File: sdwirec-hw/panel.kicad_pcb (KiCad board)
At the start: 4 copper layers, 71 x 70 mm, 272 parts, among them IC1 USB2640-HZH-02, IC2 MC74HC1G04DTT1G, J1 USB_C_Receptacle_USB2.0, J2 usd_plug, J3 Micro_SD_Card, Q1 SMMBT4403L, Q2 SMMBT4403L, U1 M24C02-RDW, U2 SPX3819M5-L-3-3, U3 TS3A27518EPW, U4 FT200XD, Y1 24Mhz

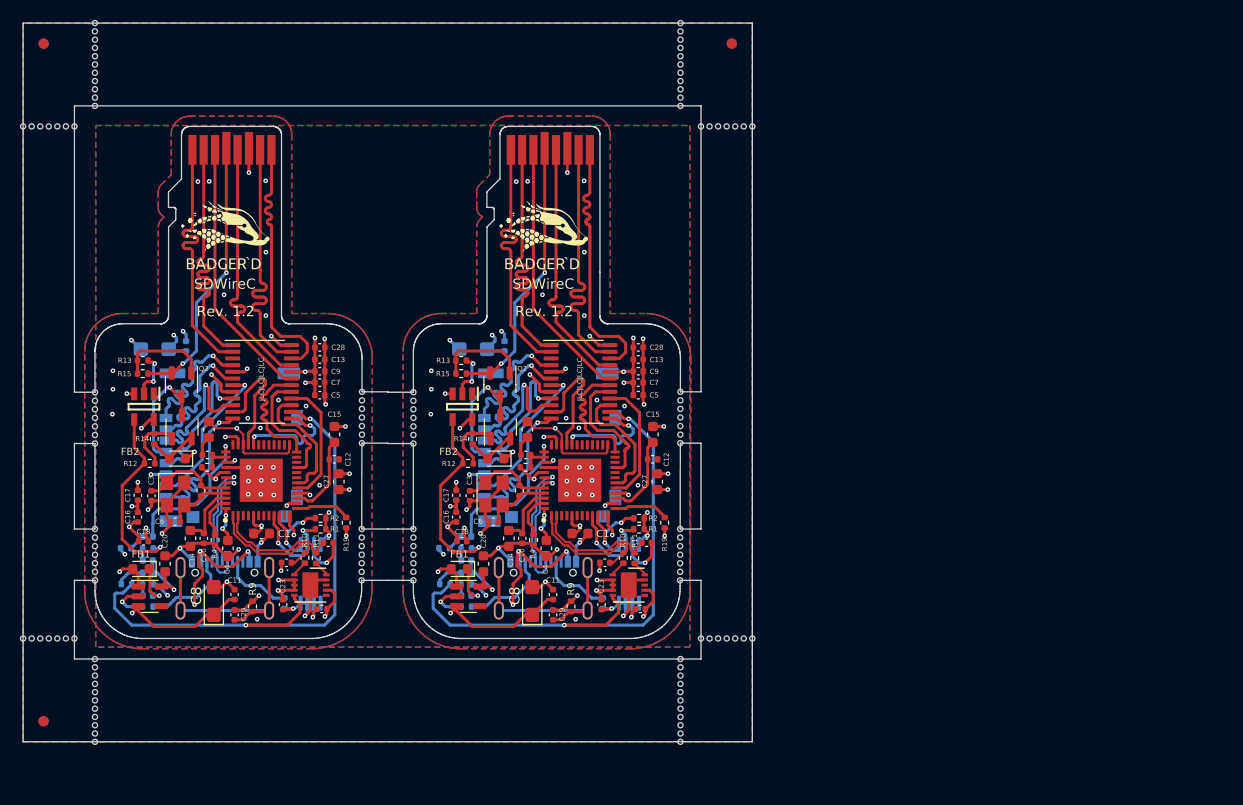
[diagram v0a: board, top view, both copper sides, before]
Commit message: Update to Rev 1.4
Signed-off-by: Talha Can Havadar <talha.can.havadar@canonical.com>
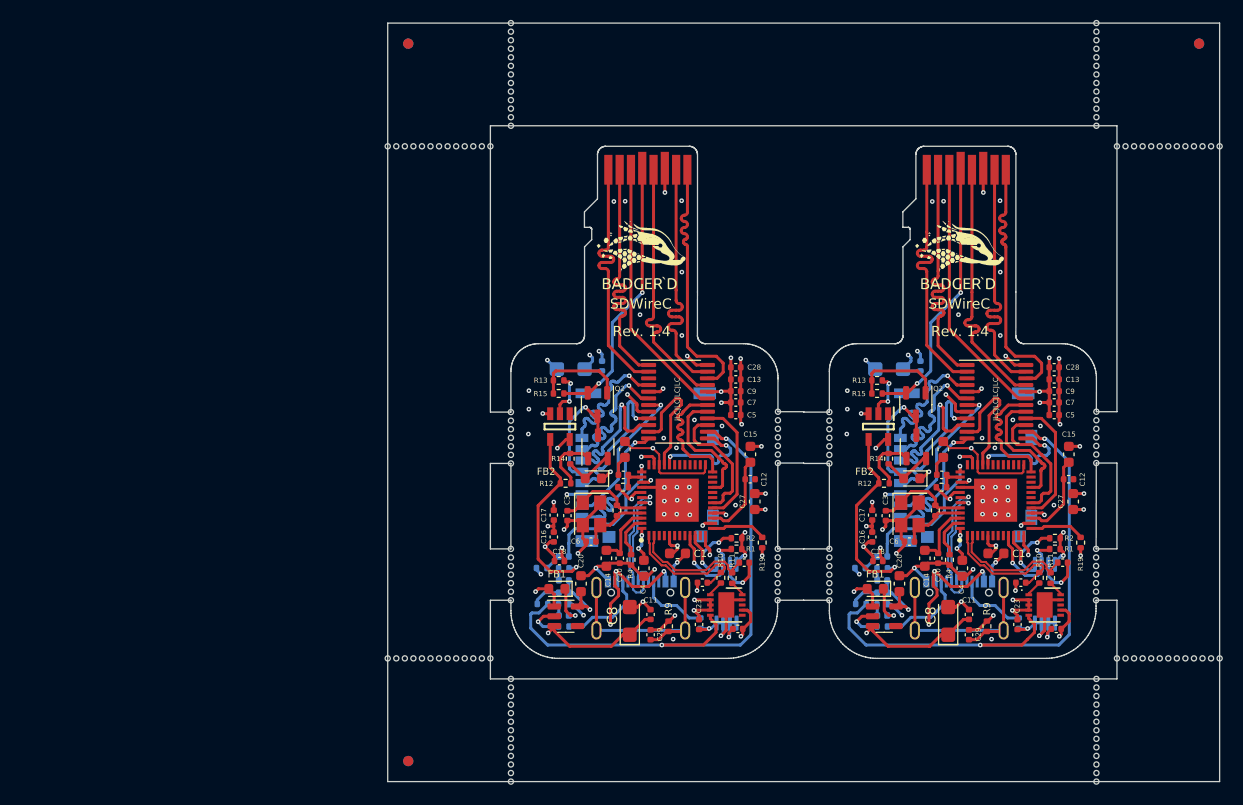
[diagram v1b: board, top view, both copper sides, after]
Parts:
- removed the C1 at (167.2, 69.7)
- removed the C1 at (136.2, 69.7)
- removed the C10 at (130.6, 70.2)
- removed the C10 at (161.6, 70.2)
- removed the C11 at (133.6, 75.7)
- removed the C11 at (164.6, 75.7)
- removed the C12 at (143.3, 62.5)
- removed the C12 at (174.3, 62.5)
- removed the C13 at (141.9, 52.8)
- removed the C13 at (172.9, 52.8)
- removed the C14 at (129.3, 70.2)
- removed the C14 at (160.3, 70.2)
- removed the C15 at (143.3, 60.1)
- removed the C15 at (174.3, 60.1)
- removed the C16 at (124.2, 68.1)
- removed the C16 at (155.2, 68.1)
- removed the C17 at (124.2, 66.0)
- removed the C17 at (155.2, 66.0)
- removed the C18 at (124.7, 70.5)
- removed the C18 at (155.7, 70.5)
- removed the C19 at (130.9, 62.1)
- removed the C19 at (162.0, 62.1)
- removed the C2 at (173.1, 77.1)
- removed the C2 at (142.1, 77.1)
- removed the C20 at (157.8, 72.7)
- removed the C20 at (126.8, 72.7)
- removed the C21 at (169.7, 72.6)
- removed the C21 at (138.6, 72.6)
- removed the C22 at (173.7, 70.6)
- removed the C22 at (142.7, 70.6)
- removed the C23 at (138.3, 76.6)
- removed the C23 at (169.3, 76.6)
- removed the C24 at (125.8, 51.8)
- removed the C24 at (156.8, 51.8)
- removed the C25 at (128.9, 51.5)
- removed the C25 at (159.9, 51.5)
- removed the C26 at (162.1, 59.6)
- removed the C26 at (131.1, 59.6)
- removed the C27 at (174.8, 64.7)
- removed the C27 at (143.7, 64.7)
- removed the C28 at (172.9, 51.6)
- removed the C28 at (141.9, 51.6)
- removed the C29 at (133.6, 77.6)
- removed the C29 at (164.6, 77.6)
- removed the C3 at (156.5, 66.0)
- removed the C3 at (125.5, 66.0)
- removed the C4 at (132.9, 71.2)
- removed the C4 at (164.0, 71.2)
- removed the C5 at (172.9, 56.2)
- removed the C5 at (141.9, 56.2)
- removed the C6 at (127.8, 68.6)
- removed the C6 at (158.8, 68.6)
- removed the C7 at (172.9, 55.0)
- removed the C7 at (141.9, 55.0)
- removed the C8 at (162.6, 76.3)
- removed the C8 at (131.6, 76.3)
- removed the C9 at (172.9, 53.9)
- removed the C9 at (141.9, 53.9)
- removed the D1 at (125.1, 75.8)
- removed the D1 at (156.2, 75.8)
- removed the D2 at (156.2, 70.0)
- removed the D2 at (125.1, 70.0)
- removed the D3 at (156.2, 73.5)
- removed the D3 at (125.1, 73.5)
- removed the D4 at (156.2, 72.3)
- removed the D4 at (125.1, 72.3)
- removed the FB1 at (155.5, 73.2)
- removed the FB1 at (124.5, 73.2)
- removed the FB2 at (159.0, 62.4)
- removed the FB2 at (128.0, 62.4)
- removed the G*** at (132.7, 40.7) (x2)
- removed the G*** at (163.7, 40.7) (x2)
- removed the IC1 at (136.2, 64.5)
- removed the IC1 at (167.2, 64.5)
- removed the IC2 at (124.8, 57.4)
- removed the IC2 at (155.8, 57.4)
- removed the J1 at (163.7, 76.1)
- removed the J1 at (132.6, 76.1)
- removed the J2 at (160.5, 32.3)
- removed the J2 at (129.5, 32.3)
- removed the J3 at (158.6, 61.3)
- removed the J3 at (127.5, 61.3)
- removed the Q1 at (159.5, 59.3)
- removed the Q1 at (128.5, 59.3)
- removed the Q2 at (128.4, 55.2)
- removed the Q2 at (159.4, 55.2)
- removed the R1 at (173.0, 69.3)
- removed the R1 at (142.0, 69.3)
- removed the R10 at (140.4, 72.1)
- removed the R10 at (171.5, 72.1)
- removed the R11 at (141.5, 72.1)
- removed the R11 at (172.6, 72.1)
- removed the R12 at (156.3, 62.9)
- removed the R12 at (125.3, 62.9)
- removed the R13 at (155.7, 52.9)
- removed the R13 at (124.6, 52.9)
- removed the R14 at (156.8, 60.5)
- removed the R14 at (125.8, 60.5)
- removed the R15 at (124.6, 54.1)
- removed the R15 at (155.7, 54.1)
- removed the R16 at (154.1, 74.6)
- removed the R16 at (123.1, 74.6)
- removed the R17 at (125.1, 71.2)
- removed the R17 at (156.2, 71.2)
- removed the R18 at (161.3, 65.5)
- removed the R18 at (130.3, 65.5)
- removed the R19 at (144.5, 68.7)
- removed the R19 at (175.5, 68.7)
- removed the R2 at (173.0, 68.2)
- removed the R2 at (142.0, 68.2)
- removed the R3 at (125.1, 74.7)
- removed the R3 at (156.2, 74.7)
- removed the R4 at (131.7, 70.3)
- removed the R4 at (162.7, 70.3)
- removed the R5 at (161.9, 63.3)
- removed the R5 at (130.9, 63.3)
- removed the R6 at (154.0, 71.1)
- removed the R6 at (123.0, 71.1)
- removed the R7 at (125.1, 76.8)
- removed the R7 at (156.2, 76.8)
- removed the R8 at (169.5, 76.5)
- removed the R8 at (138.4, 76.5)
- removed the R9 at (166.4, 76.8)
- removed the R9 at (135.3, 76.8)
- removed the REF** at (120.0, 82.7)
- removed the REF** at (177.0, 60.9)
- removed the REF** at (117.2, 30.1)
- removed the REF** at (177.0, 73.4)
- removed the REF** at (177.0, 24.8)
- removed the REF** at (177.0, 81.9)
- removed the REF** at (151.0, 60.1)
- removed the REF** at (182.3, 30.1)
- removed the REF** at (177.0, 82.7)
- removed the REF** at (182.0, 22.0) (x2)
- removed the REF** at (177.0, 69.3)
- removed the REF** at (120.0, 56.0)
- removed the REF** at (151.0, 70.1)
- removed the REF** at (120.0, 23.2)
- removed the REF** at (120.0, 74.3)
- removed the REF** at (184.0, 79.9)
- removed the REF** at (120.0, 28.1)
- removed the REF** at (177.0, 84.4)
- removed the REF** at (120.0, 83.5)
- removed the REF** at (151.0, 73.4)
- removed the REF** at (179.8, 30.1)
- removed the REF** at (120.0, 84.4)
- removed the REF** at (177.0, 20.0)
- removed the REF** at (146.0, 73.4)
- removed the REF** at (120.0, 58.5)
- removed the REF** at (177.0, 57.6)
- removed the REF** at (177.0, 24.0)
- removed the REF** at (180.7, 30.1)
- removed the REF** at (146.0, 74.3)
- removed the REF** at (120.0, 21.6)
- removed the REF** at (177.0, 27.3)
- removed the REF** at (177.0, 72.6)
- removed the REF** at (120.0, 27.3)
- removed the REF** at (120.0, 86.0)
- removed the REF** at (182.3, 79.9)
- removed the REF** at (146.0, 57.6)
- removed the REF** at (177.0, 21.6)
- removed the REF** at (133.8, 50.2)
- removed the REF** at (115.0, 22.0) (x2)
- removed the REF** at (115.0, 88.0) (x2)
- removed the REF** at (164.8, 50.2)
- removed the REF** at (177.0, 55.9)
- removed the REF** at (177.0, 89.2)
- removed the REF** at (177.0, 26.4)
- removed the REF** at (183.2, 79.9)
- removed the REF** at (120.0, 56.8)
- removed the REF** at (118.0, 30.1)
- removed the REF** at (117.2, 79.9)
- removed the REF** at (120.0, 86.8)
- removed the REF** at (146.0, 72.6)
- removed the REF** at (120.0, 81.9)
- removed the REF** at (177.0, 25.6)
- removed the REF** at (120.0, 24.8)
- removed the REF** at (177.0, 22.4)
- removed the REF** at (151.0, 71.8)
- removed the REF** at (120.0, 87.6)
- removed the REF** at (146.0, 70.1)
- removed the REF** at (120.0, 25.6)
- removed the REF** at (181.5, 79.9)
- removed the REF** at (120.0, 22.4)
- removed the REF** at (151.0, 57.6)
- removed the REF** at (177.0, 70.9)
- removed the REF** at (177.0, 86.0)
- removed the REF** at (177.0, 28.1)
- removed the REF** at (151.0, 74.3)
- removed the REF** at (114.7, 30.1)
- removed the REF** at (114.7, 79.9)
- removed the REF** at (120.0, 70.1)
- removed the REF** at (113.8, 30.1)
- removed the REF** at (120.0, 57.6)
- removed the REF** at (113.0, 79.9)
- removed the REF** at (120.0, 85.2)
- removed the REF** at (151.0, 56.8)
- removed the REF** at (179.0, 30.1)
- removed the REF** at (177.0, 85.2)
- removed the REF** at (183.2, 30.1)
- removed the REF** at (146.0, 56.7)
- removed the REF** at (120.0, 24.0)
- removed the REF** at (120.0, 59.3)
- removed the REF** at (177.0, 59.2)
- removed the REF** at (151.0, 58.5)
- removed the REF** at (177.0, 87.6)
- removed the REF** at (177.0, 58.4)
- removed the REF** at (179.8, 79.9)
- removed the REF** at (177.0, 56.7)
- removed the REF** at (120.0, 26.4)
- removed the REF** at (180.7, 79.9)
- removed the REF** at (120.0, 72.6)
- removed the REF** at (177.0, 83.5)
- removed the REF** at (177.0, 90.0)
- removed the REF** at (120.0, 60.1)
- removed the REF** at (146.0, 55.9)
- removed the REF** at (184.0, 30.1)
- removed the REF** at (177.0, 70.1)
- removed the REF** at (146.0, 70.9)
- removed the REF** at (113.0, 30.1)
- removed the REF** at (118.0, 79.9)
- removed the REF** at (146.0, 69.3)
- removed the REF** at (120.0, 89.2)
- removed the REF** at (146.0, 60.1)
- removed the REF** at (177.0, 60.1)
- removed the REF** at (181.5, 30.1)
- removed the REF** at (151.0, 56.0)
- removed the REF** at (146.0, 58.4)
- removed the REF** at (120.0, 90.0)
- removed the REF** at (151.0, 69.3)
- removed the REF** at (115.5, 30.1)
- removed the REF** at (177.0, 23.2)
- removed the REF** at (151.0, 70.9)
- removed the REF** at (120.0, 69.3)
- removed the REF** at (120.0, 20.0)
- removed the REF** at (120.0, 73.4)
- removed the REF** at (120.0, 88.4)
- removed the REF** at (146.0, 59.2)
- removed the REF** at (151.0, 72.6)
- removed the REF** at (113.8, 79.9)
- removed the REF** at (120.0, 20.8)
- removed the REF** at (177.0, 86.8)
- removed the REF** at (116.3, 30.1)
- removed the REF** at (116.3, 79.9)
- removed the REF** at (115.5, 79.9)
- removed the REF** at (177.0, 20.8)
- removed the REF** at (146.0, 60.9)
- removed the REF** at (120.0, 61.0)
- removed the REF** at (179.0, 79.9)
- removed the REF** at (120.0, 70.9)
- removed the REF** at (151.0, 61.0)
- removed the REF** at (177.0, 74.3)
- removed the REF** at (146.0, 71.8)
- removed the REF** at (177.0, 88.4)
- removed the REF** at (177.0, 71.8)
- removed the REF** at (120.0, 71.8)
- removed the REF** at (151.0, 59.3)
- removed the U1 at (172.0, 73.6)
- removed the U1 at (141.0, 73.6)
- removed the U2 at (125.3, 75.8)
- removed the U2 at (156.4, 75.8)
- removed the U3 at (167.3, 54.9)
- removed the U3 at (136.3, 54.9)
- removed the U4 at (141.0, 74.7)
- removed the U4 at (172.0, 74.7)
- removed the Y1 at (127.8, 65.9)
- removed the Y1 at (158.9, 65.9)
- added C1: 1uF, Capacitor_SMD:C_0603_1608Metric, F.Cu at (207.7, 71.7)
- added C1: 1uF, Capacitor_SMD:C_0603_1608Metric, F.Cu at (176.7, 71.7)
- added C10: 100nF, Capacitor_SMD:C_0402_1005Metric, F.Cu at (202.1, 72.1)
- added C10: 100nF, Capacitor_SMD:C_0402_1005Metric, F.Cu at (171.1, 72.1)
- added C11: 100nF / 16V, Capacitor_SMD:C_0402_1005Metric, F.Cu at (205.1, 77.6)
- added C11: 100nF / 16V, Capacitor_SMD:C_0402_1005Metric, F.Cu at (174.1, 77.6)
- added C12: 100nF, Capacitor_SMD:C_0402_1005Metric, F.Cu at (214.8, 64.4)
- added C12: 100nF, Capacitor_SMD:C_0402_1005Metric, F.Cu at (183.8, 64.4)
- added C13: 100nF, Capacitor_SMD:C_0402_1005Metric, F.Cu at (182.4, 54.7)
- added C13: 100nF, Capacitor_SMD:C_0402_1005Metric, F.Cu at (213.4, 54.7)
- added C14: 1uF, Capacitor_SMD:C_0603_1608Metric, F.Cu at (200.8, 72.1)
- added C14: 1uF, Capacitor_SMD:C_0603_1608Metric, F.Cu at (169.8, 72.1)
- added C15: 1uF, Capacitor_SMD:C_0603_1608Metric, F.Cu at (214.8, 62.0)
- added C15: 1uF, Capacitor_SMD:C_0603_1608Metric, F.Cu at (183.8, 62.0)
- added C16: 100nF, Capacitor_SMD:C_0402_1005Metric, F.Cu at (195.7, 70.0)
- added C16: 100nF, Capacitor_SMD:C_0402_1005Metric, F.Cu at (164.7, 70.0)
- added C17: 100nF, Capacitor_SMD:C_0402_1005Metric, F.Cu at (164.7, 67.9)
- added C17: 100nF, Capacitor_SMD:C_0402_1005Metric, F.Cu at (195.7, 67.9)
- added C18: 100nF / 16V, Capacitor_SMD:C_0402_1005Metric, F.Cu at (165.2, 72.4)
- added C18: 100nF / 16V, Capacitor_SMD:C_0402_1005Metric, F.Cu at (196.2, 72.4)
- added C19: 100nF, Capacitor_SMD:C_0402_1005Metric, F.Cu at (171.5, 64.0)
- added C19: 100nF, Capacitor_SMD:C_0402_1005Metric, F.Cu at (202.5, 64.0)
- added C2: 100nF, Capacitor_SMD:C_0402_1005Metric, F.Cu at (213.6, 79.0)
- added C2: 100nF, Capacitor_SMD:C_0402_1005Metric, F.Cu at (182.6, 79.0)
- added C20: 10uF, Capacitor_SMD:C_0603_1608Metric, F.Cu at (198.3, 74.6)
- added C20: 10uF, Capacitor_SMD:C_0603_1608Metric, F.Cu at (167.3, 74.6)
- added C21: 47pF, Capacitor_SMD:C_0402_1005Metric, F.Cu at (210.2, 74.5)
- added C21: 47pF, Capacitor_SMD:C_0402_1005Metric, F.Cu at (179.2, 74.5)
- added C22: 47pF, Capacitor_SMD:C_0402_1005Metric, F.Cu at (183.2, 72.5)
- added C22: 47pF, Capacitor_SMD:C_0402_1005Metric, F.Cu at (214.2, 72.5)
- added C23: 100nF, Capacitor_SMD:C_0402_1005Metric, F.Cu at (178.8, 78.6)
- added C23: 100nF, Capacitor_SMD:C_0402_1005Metric, F.Cu at (209.8, 78.6)
- added C24: 10uF, Capacitor_Tantalum_SMD:CP_EIA-3216-18_Kemet-A, B.Cu at (166.3, 53.7)
- added C24: 10uF, Capacitor_Tantalum_SMD:CP_EIA-3216-18_Kemet-A, B.Cu at (197.3, 53.7)
- added C25: 100nF, Capacitor_SMD:C_0402_1005Metric, B.Cu at (169.4, 53.4)
- added C25: 100nF, Capacitor_SMD:C_0402_1005Metric, B.Cu at (200.4, 53.4)
- added C26: 4.7uF, Capacitor_SMD:C_0603_1608Metric, F.Cu at (202.6, 61.5)
- added C26: 4.7uF, Capacitor_SMD:C_0603_1608Metric, F.Cu at (171.6, 61.5)
- added C27: 4.7uF, Capacitor_SMD:C_0603_1608Metric, F.Cu at (215.3, 66.6)
- added C27: 4.7uF, Capacitor_SMD:C_0603_1608Metric, F.Cu at (184.3, 66.6)
- added C28: 100nF, Capacitor_SMD:C_0402_1005Metric, F.Cu at (182.4, 53.5)
- added C28: 100nF, Capacitor_SMD:C_0402_1005Metric, F.Cu at (213.4, 53.5)
- added C29: 100nF, Capacitor_SMD:C_0402_1005Metric, F.Cu at (174.1, 79.6)
- added C29: 100nF, Capacitor_SMD:C_0402_1005Metric, F.Cu at (205.1, 79.6)
- added C3: 12pF ?, Capacitor_SMD:C_0402_1005Metric, F.Cu at (166.0, 68.0)
- added C3: 12pF ?, Capacitor_SMD:C_0402_1005Metric, F.Cu at (197.0, 68.0)
- added C4: 1uF, Capacitor_SMD:C_0603_1608Metric, F.Cu at (173.5, 73.1)
- added C4: 1uF, Capacitor_SMD:C_0603_1608Metric, F.Cu at (204.5, 73.1)
- added C5: 100nF, Capacitor_SMD:C_0402_1005Metric, F.Cu at (213.4, 58.2)
- added C5: 100nF, Capacitor_SMD:C_0402_1005Metric, F.Cu at (182.4, 58.2)
- added C6: 12pF ?, Capacitor_SMD:C_0402_1005Metric, F.Cu at (168.3, 70.5)
- added C6: 12pF ?, Capacitor_SMD:C_0402_1005Metric, F.Cu at (199.3, 70.5)
- added C7: 100nF, Capacitor_SMD:C_0402_1005Metric, F.Cu at (213.4, 57.0)
- added C7: 100nF, Capacitor_SMD:C_0402_1005Metric, F.Cu at (182.4, 57.0)
- added C8: 10uF, Capacitor_Tantalum_SMD:CP_EIA-3216-18_Kemet-A, F.Cu at (172.1, 78.2)
- added C8: 10uF, Capacitor_Tantalum_SMD:CP_EIA-3216-18_Kemet-A, F.Cu at (203.1, 78.2)
- added C9: 100nF, Capacitor_SMD:C_0402_1005Metric, F.Cu at (182.4, 55.9)
- added C9: 100nF, Capacitor_SMD:C_0402_1005Metric, F.Cu at (213.4, 55.9)
- added D1: Red, LED_SMD:LED_0402_1005Metric, B.Cu at (165.7, 77.7)
- added D1: Red, LED_SMD:LED_0402_1005Metric, B.Cu at (196.7, 77.7)
- added D2: Green, LED_SMD:LED_0402_1005Metric, B.Cu at (165.7, 72.0)
- added D2: Green, LED_SMD:LED_0402_1005Metric, B.Cu at (196.7, 72.0)
- added D3: Blue, LED_SMD:LED_0402_1005Metric, B.Cu at (165.7, 75.5)
- added D3: Blue, LED_SMD:LED_0402_1005Metric, B.Cu at (196.7, 75.5)
- added D4: Yellow, LED_SMD:LED_0402_1005Metric, B.Cu at (165.7, 74.3)
- added D4: Yellow, LED_SMD:LED_0402_1005Metric, B.Cu at (196.7, 74.3)
- added FB1: 150R, Diode_SMD:D_0603_1608Metric, F.Cu at (165.0, 75.1)
- added FB1: 150R, Diode_SMD:D_0603_1608Metric, F.Cu at (196.0, 75.1)
- added FB2: 150R, Diode_SMD:D_0603_1608Metric, F.Cu at (199.5, 64.3)
- added FB2: 150R, Diode_SMD:D_0603_1608Metric, F.Cu at (168.5, 64.3)
- added G***: LOGO, sdwirec:badgerd-logo-9mm, F.Cu at (173.2, 42.6)
- added G***: LOGO, sdwirec:badgerd-logo-9mm, F.Cu at (204.2, 42.6)
- added G***: LOGO, sdwirec:badgerd-logo-9mm, B.Cu at (204.2, 42.6)
- added G***: LOGO, sdwirec:badgerd-logo-9mm, B.Cu at (173.2, 42.6)
- added IC1: USB2640-HZH-02, sdwirec:QFN50P700X700X100-49N-D, F.Cu at (176.7, 66.5)
- added IC1: USB2640-HZH-02, sdwirec:QFN50P700X700X100-49N-D, F.Cu at (207.7, 66.5)
- added IC2: MC74HC1G04DTT1G, sdwirec:SOT95P275X110-5N, F.Cu at (165.3, 59.3)
- added IC2: MC74HC1G04DTT1G, sdwirec:SOT95P275X110-5N, F.Cu at (196.3, 59.3)
- added J1: USB_C_Receptacle_USB2.0, Connector_USB:USB_C_Receptacle_GCT_USB4105-xx-A_16P_TopMnt_Horizontal, B.Cu at (173.2, 78.1)
- added J1: USB_C_Receptacle_USB2.0, Connector_USB:USB_C_Receptacle_GCT_USB4105-xx-A_16P_TopMnt_Horizontal, B.Cu at (204.2, 78.1)
- added J2: usd_plug, sdwirec:usd, F.Cu at (201.0, 34.3)
- added J2: usd_plug, sdwirec:usd, F.Cu at (170.0, 34.3)
- added J3: Micro_SD_Card, sdwirec:5031821852, B.Cu at (168.1, 63.2)
- added J3: Micro_SD_Card, sdwirec:5031821852, B.Cu at (199.1, 63.2)
- added Q1: SMMBT4403L, Package_TO_SOT_SMD:SOT-23-3, F.Cu at (200.0, 61.3)
- added Q1: SMMBT4403L, Package_TO_SOT_SMD:SOT-23-3, F.Cu at (169.0, 61.3)
- added Q2: SMMBT4403L, Package_TO_SOT_SMD:SOT-23-3, F.Cu at (199.9, 57.1)
- added Q2: SMMBT4403L, Package_TO_SOT_SMD:SOT-23-3, F.Cu at (168.9, 57.1)
- added R1: 10K, Resistor_SMD:R_0402_1005Metric, F.Cu at (213.5, 71.2)
- added R1: 10K, Resistor_SMD:R_0402_1005Metric, F.Cu at (182.5, 71.2)
- added R10: 27R, Resistor_SMD:R_0402_1005Metric, F.Cu at (212.0, 74.0)
- added R10: 27R, Resistor_SMD:R_0402_1005Metric, F.Cu at (181.0, 74.0)
- added R11: 27R, Resistor_SMD:R_0402_1005Metric, F.Cu at (213.1, 74.0)
- added R11: 27R, Resistor_SMD:R_0402_1005Metric, F.Cu at (182.1, 74.0)
- added R12: 1.5K, Resistor_SMD:R_0402_1005Metric, F.Cu at (196.8, 64.8)
- added R12: 1.5K, Resistor_SMD:R_0402_1005Metric, F.Cu at (165.8, 64.8)
- added R13: 1.5K, Resistor_SMD:R_0402_1005Metric, F.Cu at (165.2, 54.8)
- added R13: 1.5K, Resistor_SMD:R_0402_1005Metric, F.Cu at (196.2, 54.8)
- added R14: 10K, Resistor_SMD:R_0402_1005Metric, F.Cu at (197.3, 62.4)
- added R14: 10K, Resistor_SMD:R_0402_1005Metric, F.Cu at (166.3, 62.4)
- added R15: 10K, Resistor_SMD:R_0402_1005Metric, F.Cu at (196.2, 56.1)
- added R15: 10K, Resistor_SMD:R_0402_1005Metric, F.Cu at (165.2, 56.1)
- added R16: 1.5K, Resistor_SMD:R_0402_1005Metric, B.Cu at (194.6, 76.6)
- added R16: 1.5K, Resistor_SMD:R_0402_1005Metric, B.Cu at (163.6, 76.6)
- added R17: 1.5K, Resistor_SMD:R_0402_1005Metric, B.Cu at (196.7, 73.1)
- added R17: 1.5K, Resistor_SMD:R_0402_1005Metric, B.Cu at (165.7, 73.1)
- added R18: 1M, Resistor_SMD:R_0402_1005Metric, F.Cu at (170.8, 67.5)
- added R18: 1M, Resistor_SMD:R_0402_1005Metric, F.Cu at (201.8, 67.5)
- added R19: 0R, Resistor_SMD:R_0402_1005Metric, F.Cu at (216.0, 70.6)
- added R19: 0R, Resistor_SMD:R_0402_1005Metric, F.Cu at (185.0, 70.6)
- added R2: 10K, Resistor_SMD:R_0402_1005Metric, F.Cu at (213.5, 70.2)
- added R2: 10K, Resistor_SMD:R_0402_1005Metric, F.Cu at (182.5, 70.2)
- added R3: 1.5K, Resistor_SMD:R_0402_1005Metric, B.Cu at (165.7, 76.6)
- added R3: 1.5K, Resistor_SMD:R_0402_1005Metric, B.Cu at (196.7, 76.6)
- added R4: 12K, Resistor_SMD:R_0402_1005Metric, F.Cu at (172.2, 72.3)
- added R4: 12K, Resistor_SMD:R_0402_1005Metric, F.Cu at (203.2, 72.3)
- added R5: 10K, Resistor_SMD:R_0402_1005Metric, F.Cu at (171.4, 65.2)
- added R5: 10K, Resistor_SMD:R_0402_1005Metric, F.Cu at (202.4, 65.2)
- added R6: 1.5K, Resistor_SMD:R_0402_1005Metric, B.Cu at (194.5, 73.1)
- added R6: 1.5K, Resistor_SMD:R_0402_1005Metric, B.Cu at (163.5, 73.1)
- added R7: 5.1K, Resistor_SMD:R_0402_1005Metric, B.Cu at (196.7, 78.8)
- added R7: 5.1K, Resistor_SMD:R_0402_1005Metric, B.Cu at (165.7, 78.8)
- added R8: 5.1K, Resistor_SMD:R_0402_1005Metric, B.Cu at (210.0, 78.5)
- added R8: 5.1K, Resistor_SMD:R_0402_1005Metric, B.Cu at (179.0, 78.5)
- added R9: 10K, Resistor_SMD:R_0402_1005Metric, F.Cu at (175.9, 78.8)
- added R9: 10K, Resistor_SMD:R_0402_1005Metric, F.Cu at (206.9, 78.8)
- added REF**: NPTH, NPTH, F.Cu at (217.5, 71.2)
- added REF**: NPTH, NPTH, F.Cu at (151.8, 32.0)
- added REF**: NPTH, NPTH, F.Cu at (160.5, 75.4)
- added REF**: NPTH, NPTH, F.Cu at (217.5, 72.0)
- added REF**: NPTH, NPTH, F.Cu at (160.5, 86.4)
- added REF**: NPTH, NPTH, F.Cu at (156.8, 81.9)
- added REF**: NPTH, NPTH, F.Cu at (153.5, 81.9)
- added REF**: NPTH, NPTH, F.Cu at (160.5, 74.5)
- added REF**: NPTH, NPTH, F.Cu at (217.5, 73.7)
- added REF**: NPTH, NPTH, F.Cu at (186.5, 71.2)
- added REF**: NPTH, NPTH, F.Cu at (191.5, 60.4)
- added REF**: NPTH, NPTH, F.Cu at (158.5, 81.9)
- added REF**: NPTH, NPTH, F.Cu at (217.5, 90.5)
- added REF**: NPTH, NPTH, F.Cu at (160.5, 23.3)
- added REF**: NPTH, NPTH, F.Cu at (221.2, 81.9)
- added REF**: Fiducial, Fiducial, F.Cu at (150.5, 91.9)
- added REF**: NPTH, NPTH, F.Cu at (160.5, 26.7)
- added REF**: NPTH, NPTH, F.Cu at (217.5, 57.9)
- added REF**: NPTH, NPTH, F.Cu at (186.5, 76.2)
- added REF**: NPTH, NPTH, F.Cu at (217.5, 74.5)
- added REF**: NPTH, NPTH, F.Cu at (160.5, 29.2)
- added REF**: NPTH, NPTH, F.Cu at (155.2, 81.9)
- added REF**: NPTH, NPTH, F.Cu at (222.9, 81.9)
- added REF**: NPTH, NPTH, F.Cu at (160.5, 61.2)
- added REF**: NPTH, NPTH, F.Cu at (157.7, 81.9)
- added REF**: NPTH, NPTH, F.Cu at (151.0, 81.9)
- added REF**: NPTH, NPTH, F.Cu at (217.5, 62.0)
- added REF**: NPTH, NPTH, F.Cu at (222.0, 81.9)
- added REF**: NPTH, NPTH, F.Cu at (186.5, 59.5)
- added REF**: NPTH, NPTH, F.Cu at (227.0, 81.9)
- added REF**: NPTH, NPTH, F.Cu at (217.5, 58.7)
- added REF**: NPTH, NPTH, F.Cu at (223.7, 32.0)
- added REF**: NPTH, NPTH, F.Cu at (223.7, 81.9)
- added REF**: NPTH, NPTH, F.Cu at (152.7, 81.9)
- added REF**: NPTH, NPTH, F.Cu at (152.7, 32.0)
- added REF**: NPTH, NPTH, F.Cu at (160.5, 25.8)
- added REF**: NPTH, NPTH, F.Cu at (160.5, 72.0)
- added REF**: NPTH, NPTH, F.Cu at (222.9, 32.0)
- added REF**: NPTH, NPTH, F.Cu at (217.5, 92.2)
- added REF**: NPTH, NPTH, F.Cu at (191.5, 73.7)
- added REF**: NPTH, NPTH, F.Cu at (160.5, 87.2)
- added REF**: NPTH, NPTH, F.Cu at (153.5, 32.0)
- added REF**: NPTH, NPTH, F.Cu at (160.5, 71.2)
- added REF**: NPTH, NPTH, F.Cu at (150.2, 32.0)
- added REF**: NPTH, NPTH, F.Cu at (186.5, 60.4)
- added REF**: NPTH, NPTH, F.Cu at (150.2, 81.9)
- added REF**: NPTH, NPTH, F.Cu at (186.5, 62.9)
- added REF**: NPTH, NPTH, F.Cu at (160.5, 25.0)
- added REF**: NPTH, NPTH, F.Cu at (222.0, 32.0)
- added REF**: NPTH, NPTH, F.Cu at (191.5, 61.2)
- added REF**: NPTH, NPTH, F.Cu at (160.5, 84.7)
- added REF**: NPTH, NPTH, F.Cu at (225.4, 81.9)
- added REF**: NPTH, NPTH, F.Cu at (191.5, 71.2)
- added REF**: NPTH, NPTH, F.Cu at (217.5, 62.9)
- added REF**: NPTH, NPTH, F.Cu at (158.5, 32.0)
- added REF**: NPTH, NPTH, F.Cu at (221.2, 32.0)
- added REF**: NPTH, NPTH, F.Cu at (160.5, 73.7)
- added REF**: NPTH, NPTH, F.Cu at (186.5, 72.9)
- added REF**: NPTH, NPTH, F.Cu at (217.5, 29.2)
- added REF**: NPTH, NPTH, F.Cu at (186.5, 62.0)
- added REF**: NPTH, NPTH, F.Cu at (226.2, 32.0)
- added REF**: NPTH, NPTH, F.Cu at (160.5, 76.2)
- added REF**: NPTH, NPTH, F.Cu at (217.5, 22.5)
- added REF**: NPTH, NPTH, F.Cu at (220.4, 81.9)
- added REF**: NPTH, NPTH, F.Cu at (217.5, 76.2)
- added REF**: NPTH, NPTH, F.Cu at (217.5, 25.0)
- added REF**: NPTH, NPTH, F.Cu at (160.5, 24.2)
- added REF**: NPTH, NPTH, F.Cu at (191.5, 72.0)
- added REF**: NPTH, NPTH, F.Cu at (148.5, 81.9)
- added REF**: NPTH, NPTH, F.Cu at (191.5, 74.5)
- added REF**: NPTH, NPTH, F.Cu at (228.7, 32.0)
- added REF**: NPTH, NPTH, F.Cu at (160.5, 92.2)
- added REF**: Fiducial, Fiducial, B.Cu at (150.5, 22.0)
- added REF**: ESD-Logo_6.6x6mm_SilkScreen, Symbol:ESD-Logo_6.6x6mm_SilkScreen, B.Cu at (174.3, 52.1)
- added REF**: Fiducial, Fiducial, B.Cu at (150.5, 91.9)
- added REF**: Fiducial, Fiducial, B.Cu at (227.5, 22.0)
- added REF**: ESD-Logo_6.6x6mm_SilkScreen, Symbol:ESD-Logo_6.6x6mm_SilkScreen, B.Cu at (205.4, 52.1)
- added REF**: NPTH, NPTH, F.Cu at (149.3, 81.9)
- added REF**: NPTH, NPTH, F.Cu at (225.4, 32.0)
- added REF**: NPTH, NPTH, F.Cu at (160.5, 58.7)
- added REF**: NPTH, NPTH, F.Cu at (160.5, 88.0)
- added REF**: NPTH, NPTH, F.Cu at (191.5, 59.6)
- added REF**: NPTH, NPTH, F.Cu at (219.5, 32.0)
- added REF**: NPTH, NPTH, F.Cu at (217.5, 72.9)
- added REF**: NPTH, NPTH, F.Cu at (224.5, 32.0)
- added REF**: NPTH, NPTH, F.Cu at (227.9, 81.9)
- added REF**: NPTH, NPTH, F.Cu at (217.5, 88.9)
- added REF**: NPTH, NPTH, F.Cu at (217.5, 85.5)
- added REF**: NPTH, NPTH, F.Cu at (186.5, 61.2)
- added REF**: NPTH, NPTH, F.Cu at (155.2, 32.0)
- added REF**: NPTH, NPTH, F.Cu at (160.5, 83.9)
- added REF**: NPTH, NPTH, F.Cu at (160.5, 60.4)
- added REF**: NPTH, NPTH, F.Cu at (160.5, 20.0)
- added REF**: NPTH, NPTH, F.Cu at (217.5, 26.7)
- added REF**: NPTH, NPTH, F.Cu at (160.5, 21.7)
- added REF**: NPTH, NPTH, F.Cu at (160.5, 27.5)
- added REF**: NPTH, NPTH, F.Cu at (217.5, 20.8)
- added REF**: NPTH, NPTH, F.Cu at (160.5, 57.9)
- added REF**: Fiducial, Fiducial, F.Cu at (227.5, 22.0)
- added REF**: NPTH, NPTH, F.Cu at (217.5, 60.4)
- added REF**: NPTH, NPTH, F.Cu at (186.5, 73.7)
- added REF**: NPTH, NPTH, F.Cu at (217.5, 93.9)
- added REF**: NPTH, NPTH, F.Cu at (160.5, 28.3)
- added REF**: NPTH, NPTH, F.Cu at (217.5, 25.8)
- added REF**: NPTH, NPTH, F.Cu at (160.5, 89.7)
- added REF**: NPTH, NPTH, F.Cu at (151.0, 32.0)
- added REF**: NPTH, NPTH, F.Cu at (229.5, 32.0)
- added REF**: NPTH, NPTH, F.Cu at (220.4, 32.0)
- added REF**: NPTH, NPTH, F.Cu at (217.5, 30.0)
- added REF**: NPTH, NPTH, F.Cu at (217.5, 86.4)
- added REF**: Fiducial, Fiducial, F.Cu at (150.5, 22.0)
- added REF**: NPTH, NPTH, F.Cu at (156.0, 32.0)
- added REF**: NPTH, NPTH, F.Cu at (217.5, 83.9)
- added REF**: NPTH, NPTH, F.Cu at (224.5, 81.9)
- added REF**: NPTH, NPTH, F.Cu at (186.5, 57.9)
- added REF**: NPTH, NPTH, F.Cu at (191.5, 58.7)
- added REF**: NPTH, NPTH, F.Cu at (160.5, 62.9)
- added REF**: NPTH, NPTH, F.Cu at (160.5, 72.9)
- added REF**: NPTH, NPTH, F.Cu at (217.5, 84.7)
- added REF**: NPTH, NPTH, F.Cu at (149.3, 32.0)
- added REF**: NPTH, NPTH, F.Cu at (160.5, 85.5)
- added REF**: NPTH, NPTH, F.Cu at (217.5, 75.4)
- added REF**: NPTH, NPTH, F.Cu at (217.5, 87.2)
- added REF**: NPTH, NPTH, F.Cu at (160.5, 91.4)
- added REF**: NPTH, NPTH, F.Cu at (217.5, 27.5)
- added REF**: NPTH, NPTH, F.Cu at (217.5, 88.0)
- added REF**: NPTH, NPTH, F.Cu at (186.5, 58.7)
- added REF**: NPTH, NPTH, F.Cu at (191.5, 62.1)
- added REF**: NPTH, NPTH, F.Cu at (217.5, 21.7)
- added REF**: NPTH, NPTH, F.Cu at (148.5, 32.0)
- added REF**: NPTH, NPTH, F.Cu at (227.0, 32.0)
- added REF**: NPTH, NPTH, F.Cu at (217.5, 61.2)
- added REF**: NPTH, NPTH, F.Cu at (229.5, 81.9)
- added REF**: NPTH, NPTH, F.Cu at (160.5, 93.0)
- added REF**: NPTH, NPTH, F.Cu at (191.5, 76.2)
- added REF**: NPTH, NPTH, F.Cu at (160.5, 30.0)
- added REF**: NPTH, NPTH, F.Cu at (154.3, 32.0)
- added REF**: NPTH, NPTH, F.Cu at (217.5, 28.3)
- added REF**: NPTH, NPTH, F.Cu at (217.5, 59.5)
- added REF**: NPTH, NPTH, F.Cu at (156.8, 32.0)
- added REF**: NPTH, NPTH, F.Cu at (186.5, 72.0)
- added REF**: NPTH, NPTH, F.Cu at (191.5, 72.9)
- added REF**: NPTH, NPTH, F.Cu at (227.9, 32.0)
- added REF**: NPTH, NPTH, F.Cu at (160.5, 22.5)
- added REF**: NPTH, NPTH, F.Cu at (219.5, 81.9)
- added REF**: NPTH, NPTH, F.Cu at (217.5, 20.0)
- added REF**: NPTH, NPTH, F.Cu at (191.5, 75.4)
- added REF**: NPTH, NPTH, F.Cu at (186.5, 74.5)
- added REF**: NPTH, NPTH, F.Cu at (160.5, 90.5)
- added REF**: NPTH, NPTH, F.Cu at (191.5, 57.9)
- added REF**: NPTH, NPTH, F.Cu at (156.0, 81.9)
- added REF**: NPTH, NPTH, F.Cu at (160.5, 88.9)
- added REF**: NPTH, NPTH, F.Cu at (160.5, 62.1)
- added REF**: NPTH, NPTH, F.Cu at (217.5, 89.7)
- added REF**: NPTH, NPTH, F.Cu at (160.5, 59.6)
- added REF**: NPTH, NPTH, F.Cu at (217.5, 23.3)
- added REF**: NPTH, NPTH, F.Cu at (154.3, 81.9)
- added REF**: NPTH, NPTH, F.Cu at (217.5, 93.0)
- added REF**: NPTH, NPTH, F.Cu at (191.5, 62.9)
- added REF**: NPTH, NPTH, F.Cu at (186.5, 75.4)
- added REF**: NPTH, NPTH, F.Cu at (157.7, 32.0)
- added REF**: NPTH, NPTH, F.Cu at (217.5, 24.2)
- added REF**: NPTH, NPTH, F.Cu at (160.5, 93.9)
- added REF**: NPTH, NPTH, F.Cu at (228.7, 81.9)
- added REF**: NPTH, NPTH, F.Cu at (160.5, 20.8)
- added REF**: NPTH, NPTH, F.Cu at (217.5, 91.4)
- added REF**: NPTH, NPTH, F.Cu at (151.8, 81.9)
- added REF**: NPTH, NPTH, F.Cu at (226.2, 81.9)
- added U1: M24C02-RDW, Package_SO:TSSOP-8_4.4x3mm_P0.65mm, B.Cu at (212.5, 75.6)
- added U1: M24C02-RDW, Package_SO:TSSOP-8_4.4x3mm_P0.65mm, B.Cu at (181.5, 75.6)
- added U2: SPX3819M5-L-3-3, Package_TO_SOT_SMD:SOT-23-5, F.Cu at (165.9, 77.8)
- added U2: SPX3819M5-L-3-3, Package_TO_SOT_SMD:SOT-23-5, F.Cu at (196.9, 77.8)
- added U3: TS3A27518EPW, Package_SO:TSSOP-24_4.4x7.8mm_P0.65mm, F.Cu at (207.8, 56.9)
- added U3: TS3A27518EPW, Package_SO:TSSOP-24_4.4x7.8mm_P0.65mm, F.Cu at (176.8, 56.9)
- added U4: FT200XD, Package_DFN_QFN:DFN-10-1EP_3x3mm_P0.5mm_EP1.55x2.48mm, F.Cu at (181.5, 76.7)
- added U4: FT200XD, Package_DFN_QFN:DFN-10-1EP_3x3mm_P0.5mm_EP1.55x2.48mm, F.Cu at (212.5, 76.7)
- added Y1: 24Mhz, Crystal:Crystal_SMD_3225-4Pin_3.2x2.5mm, F.Cu at (168.4, 67.8)
- added Y1: 24Mhz, Crystal:Crystal_SMD_3225-4Pin_3.2x2.5mm, F.Cu at (199.4, 67.8)
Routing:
- net +3V3: track 330.0 -> 0.00 mm, vias 42 -> 0
- net /MUX_SELECTOR: track 172.7 -> 0.00 mm, vias 10 -> 0
- net GND: track 165.6 -> 0.00 mm, vias 106 -> 0
- net Board_0-+3V3: track 0.00 -> 165.0 mm, vias 0 -> 21
- net Board_1-+3V3: track 0.00 -> 165.0 mm, vias 0 -> 21
- net Board_1-/MUX_SELECTOR: track 0.00 -> 86.3 mm, vias 0 -> 5
- net Board_0-/MUX_SELECTOR: track 0.00 -> 86.3 mm, vias 0 -> 5
- net Board_0-GND: track 0.00 -> 82.8 mm, vias 0 -> 53
- net Board_1-GND: track 0.00 -> 82.8 mm, vias 0 -> 53
- net /SD_nCD: track 66.3 -> 0.00 mm, vias 4 -> 0
- net /VDD_DEVICE: track 53.2 -> 0.00 mm, vias 4 -> 0
- net /dSD_CMD: track 51.5 -> 0.00 mm
- net /dSD_DAT1: track 51.5 -> 0.00 mm
- net /dSD_DAT2: track 51.4 -> 0.00 mm
- net /dSD_DAT3: track 51.4 -> 0.00 mm
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- removed copper zone on B.Cu, net (none)
- removed copper zone on F.Cu, net (none)
- removed copper zone on In1.Cu, net (none)
- removed copper zone on In2.Cu, net (none)
- removed copper zone on B.Cu, net GND
- removed copper zone on F.Cu, net GND
- removed copper zone on In1.Cu, net GND
- removed copper zone on In2.Cu, net GND
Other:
- board size 71 x 70 mm -> 81 x 73.9 mm
- board text added: "+"
- board text added: "Rev. 1.4"
- board text removed: "Rev. 1.2"
